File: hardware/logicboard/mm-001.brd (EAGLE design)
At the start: 91 x 57 mm, 31 parts, among them IC1 74ALS05N, IC2 LTC485N, IC3 LTC485N, J0 DC5V, J7 DIN5, J8 DIN5, J9 DIN5, X7 NELTRON-7810-XPXC, X9 NELTRON-7810-XPXC

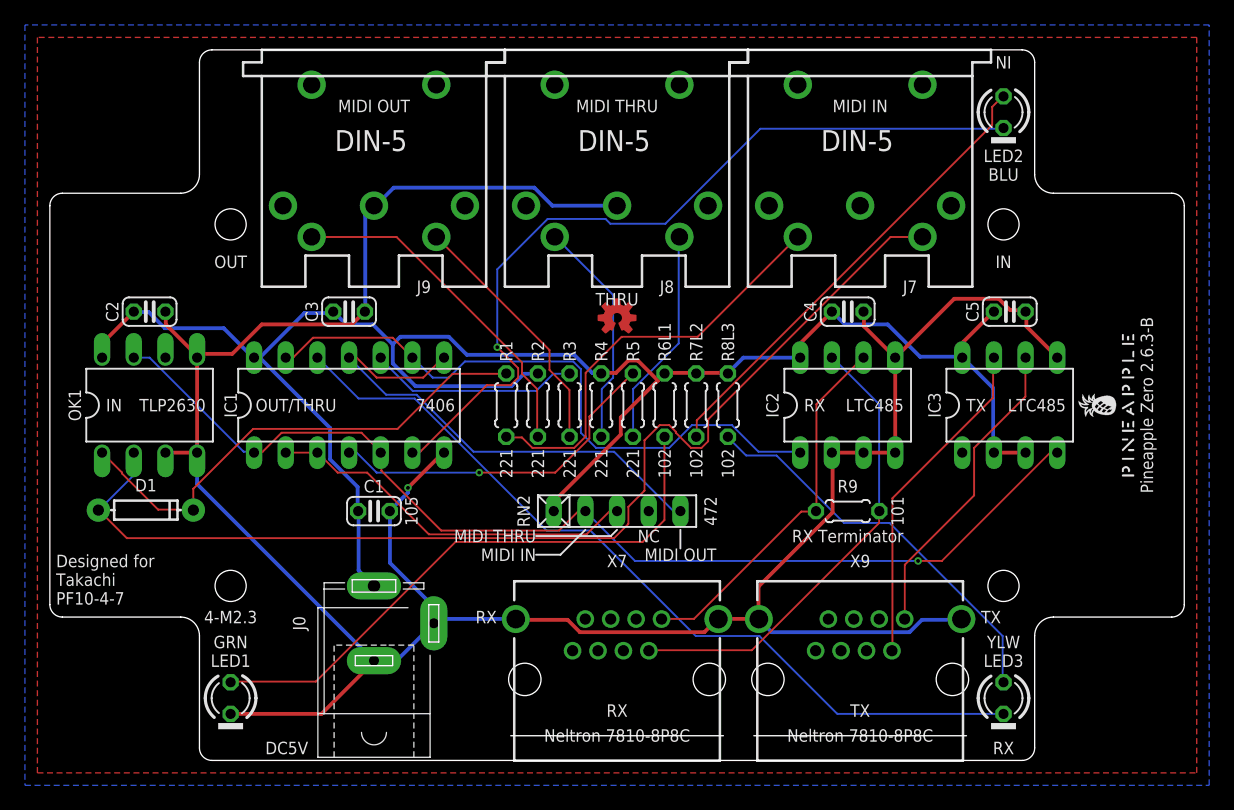
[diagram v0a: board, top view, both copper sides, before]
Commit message: Trying to fit in to the new platform.
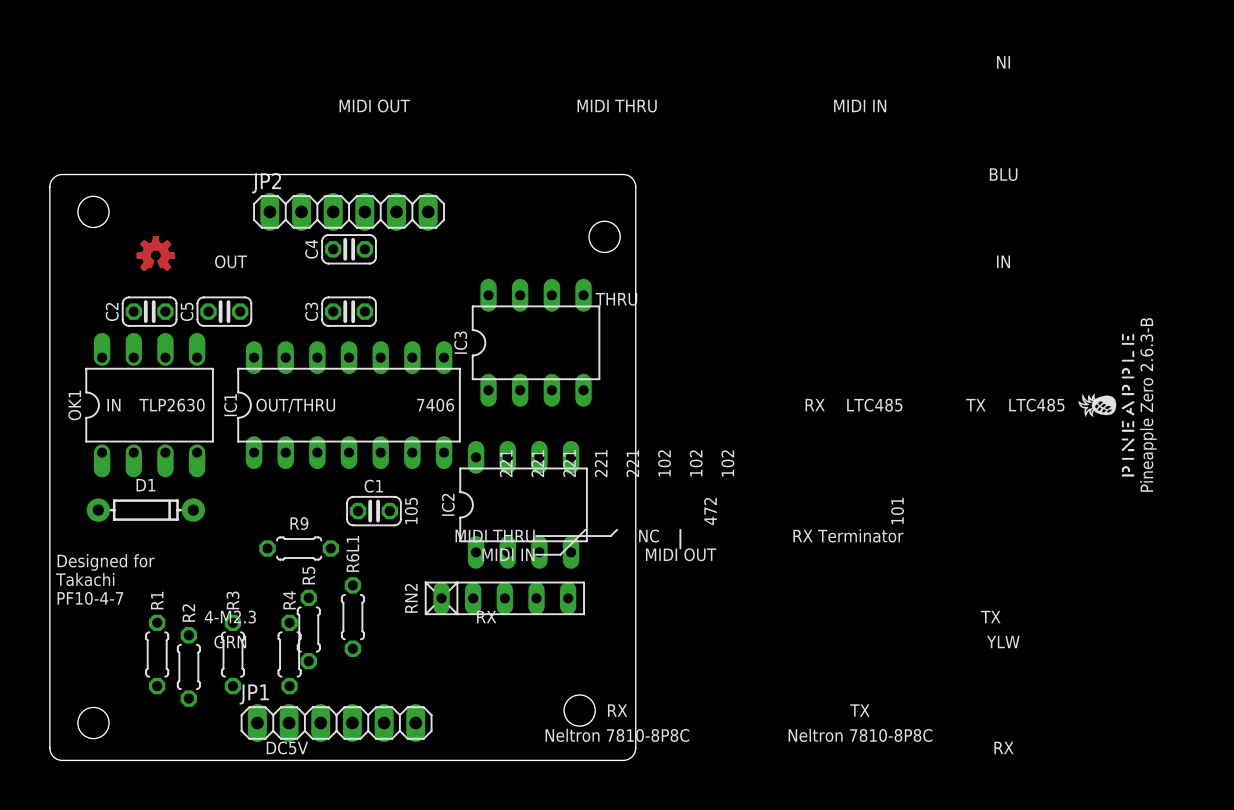
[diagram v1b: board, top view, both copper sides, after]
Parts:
- removed J0: DC5V, con-jack:SPC4077
- removed J7, J8, J9: DIN5, SparkFun-Connectors:DIN5-RA-PTH
- removed LED1: BLUE, led:LED3MM
- removed LED2, LED3: YELLOW, led:LED3MM
- removed R7L2, R8L3: 1k, rcl:0204/5
- removed X7, X9: NELTRON-7810-XPXC, con-rj45:NELTRON-7810-XPXC-FOOTPRINT
- added JP1, JP2: (no value), pinhead:1X06
- moved C5 63.0 mm to (14.0, 36.0)
- moved R9 44.1 mm to (20.0, 17.0)
- moved C4 40.3 mm to (24.0, 41.0)
- moved IC3 38.3 mm to (39.0, 33.5)
- moved LOGO1 37.3 mm to (8.50, 40.5)
- moved R2 35.0 mm to (11.2, 7.50)
- moved R1 34.4 mm to (8.61, 8.50)
- moved R3 33.6 mm to (14.7, 8.50)
- moved R4 32.0 mm to (19.2, 8.50)
- moved R5 31.6 mm to (20.8, 10.5)
- moved R6L1 30.2 mm to (24.3, 11.5)
- moved IC2 27.2 mm to (38.0, 20.5)
- moved RN2 11.4 mm to (36.5, 13.0)
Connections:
- removed net MTRTN: J8.5, R5.1
- removed net MTSND: J8.4, R4.1
- removed net N$1: IC1.6, LED2.K
- removed net N$2: LED3.A, R8L3.1
- removed net N$3: IC1.12, LED3.K
- removed net N$5: LED2.A, R7L2.1
- net GND: now also JP1.1, JP2.1; no longer J0.1, J0.2, J8.2, J9.2, LED1.K, X7.S1, X7.S2, X9.S1, X9.S2
- net MIRTN: now also JP1.4; no longer J7.5
- net MISND: now also JP1.3; no longer J7.4
- net MORTN: now also JP1.6; no longer J9.5
- net MOSND: now also JP1.5; no longer J9.4
- net N$4: now also JP2.2; no longer LED1.A
- net RX+: now also JP2.5; no longer X7.1
- net RX-: now also JP2.6; no longer X7.2
- net TX+: now also JP2.3; no longer X9.1
- net TX-: now also JP2.4; no longer X9.2
- net VCC: now also JP1.2; no longer J0.3, R7L2.2, R8L3.2
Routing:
- net GND: track 213.7 -> 0.00 mm, vias 1 -> 0
- net VCC: track 149.3 -> 0.00 mm
- net MIRTN: track 88.6 -> 0.00 mm
- net TX: track 88.0 -> 0.00 mm, vias 1 -> 0
- net N$3: track 66.9 -> 0.00 mm
- net N$1: track 66.0 -> 0.00 mm, vias 1 -> 0
- net RX: track 51.3 -> 0.00 mm
- net N$4: track 46.9 -> 0.00 mm
- net NMIDIOUT: track 40.6 -> 0.00 mm
- net MIDIIN: track 39.9 -> 0.00 mm
- net RX-: track 37.6 -> 0.00 mm
- net N$5: track 37.6 -> 0.00 mm
- net MISND: track 33.8 -> 0.00 mm
- net N$2: track 32.4 -> 0.00 mm
- net NMIDITHRU: track 30.1 -> 0.00 mm
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- removed copper zone on layer 1, net GND
- removed copper zone on layer 16, net GND
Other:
- board size 91 x 57 mm -> 47 x 47 mm
